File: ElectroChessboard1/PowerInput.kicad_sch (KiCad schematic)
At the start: 14 parts, among them J2 TYPE-C-31-M-12, U3 FT232RL

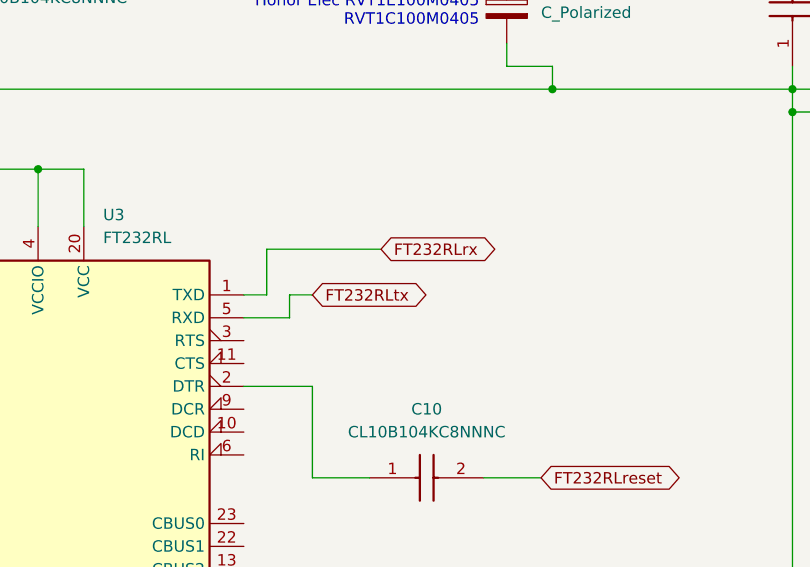
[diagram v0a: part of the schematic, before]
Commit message: Revert last commit
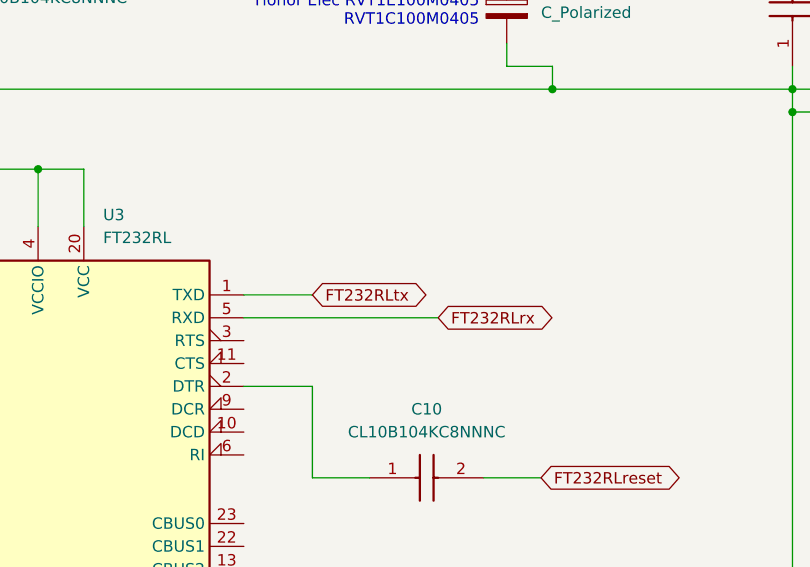
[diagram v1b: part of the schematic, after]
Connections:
- net FT232RLrx: now also U3.5 (RXD); no longer U3.1 (TXD)
- net FT232RLtx: now also U3.1 (TXD); no longer U3.5 (RXD)
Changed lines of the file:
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@@
+	(wire
+		(pts
+			(xy 127 85.09) (xy 148.59 85.09)
+		)
+		(stroke
+			(width 0)
+			(type default)
+		)
+	)
 	(wire
 		(pts
@@
 	(wire
 		(pts
-			(xy 134.62 82.55) (xy 132.08 82.55)
-		)
-		(stroke
-			(width 0)
-			(type default)
-		)
-	)
-	(wire
-		(pts
 			(xy 74.93 109.22) (xy 74.93 127)
 		)
@@
 	(wire
 		(pts
-			(xy 132.08 82.55) (xy 132.08 85.09)
-		)
-		(stroke
-			(width 0)
-			(type default)
-		)
-	)
-	(wire
-		(pts
 			(xy 63.5 132.08) (xy 71.12 132.08)
 		)
@@
 	(wire
 		(pts
-			(xy 129.54 77.47) (xy 129.54 82.55)
-		)
-		(stroke
-			(width 0)
-			(type default)
-		)
-	)
-	(wire
-		(pts
 			(xy 21.59 156.21) (xy 31.75 156.21)
 		)
@@
 	(wire
 		(pts
-			(xy 142.24 77.47) (xy 129.54 77.47)
-		)
-		(stroke
-			(width 0)
-			(type default)
-		)
-	)
-	(wire
-		(pts
 			(xy 67.31 39.37) (xy 92.71 39.37)
 		)
@@
 	(wire
 		(pts
-			(xy 132.08 85.09) (xy 127 85.09)
-		)
-		(stroke
-			(width 0)
-			(type default)
-		)
-	)
-	(wire
-		(pts
 			(xy 106.68 128.27) (xy 109.22 128.27)
 		)
@@
 	(wire
 		(pts
+			(xy 127 82.55) (xy 134.62 82.55)
+		)
+		(stroke
+			(width 0)
+			(type default)
+		)
+	)
+	(wire
+		(pts
 			(xy 67.31 146.05) (xy 67.31 139.7)
-		)
-		(stroke
-			(width 0)
-			(type default)
-		)
-	)
-	(wire
-		(pts
-			(xy 129.54 82.55) (xy 127 82.55)
 		)
 		(stroke
@@
 	(global_label "FT232RLrx"
 		(shape bidirectional)
-		(at 142.24 77.47 0)
+		(at 148.59 85.09 0)
 		(fields_autoplaced yes)
 		(effects
@@
 		)
 		(property "Intersheetrefs" "${INTERSHEET_REFS}"
-			(at 156.1336 77.47 0)
+			(at 162.4836 85.09 0)
 			(effects
 				(font
